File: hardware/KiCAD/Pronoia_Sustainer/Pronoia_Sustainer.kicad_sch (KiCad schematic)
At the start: 0 parts

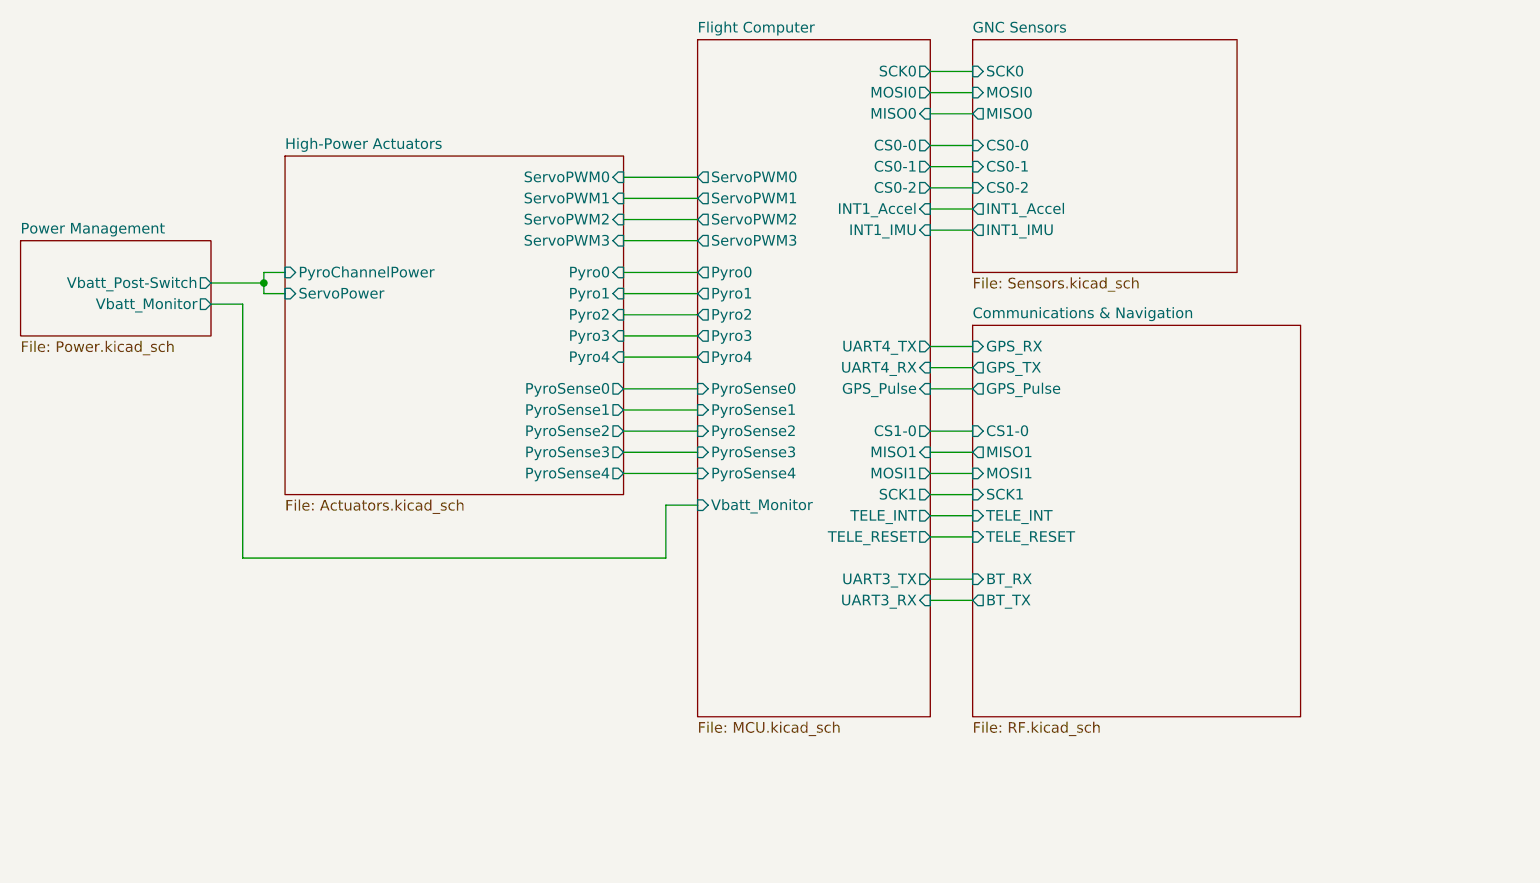
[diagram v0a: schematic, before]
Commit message: updated Schematics
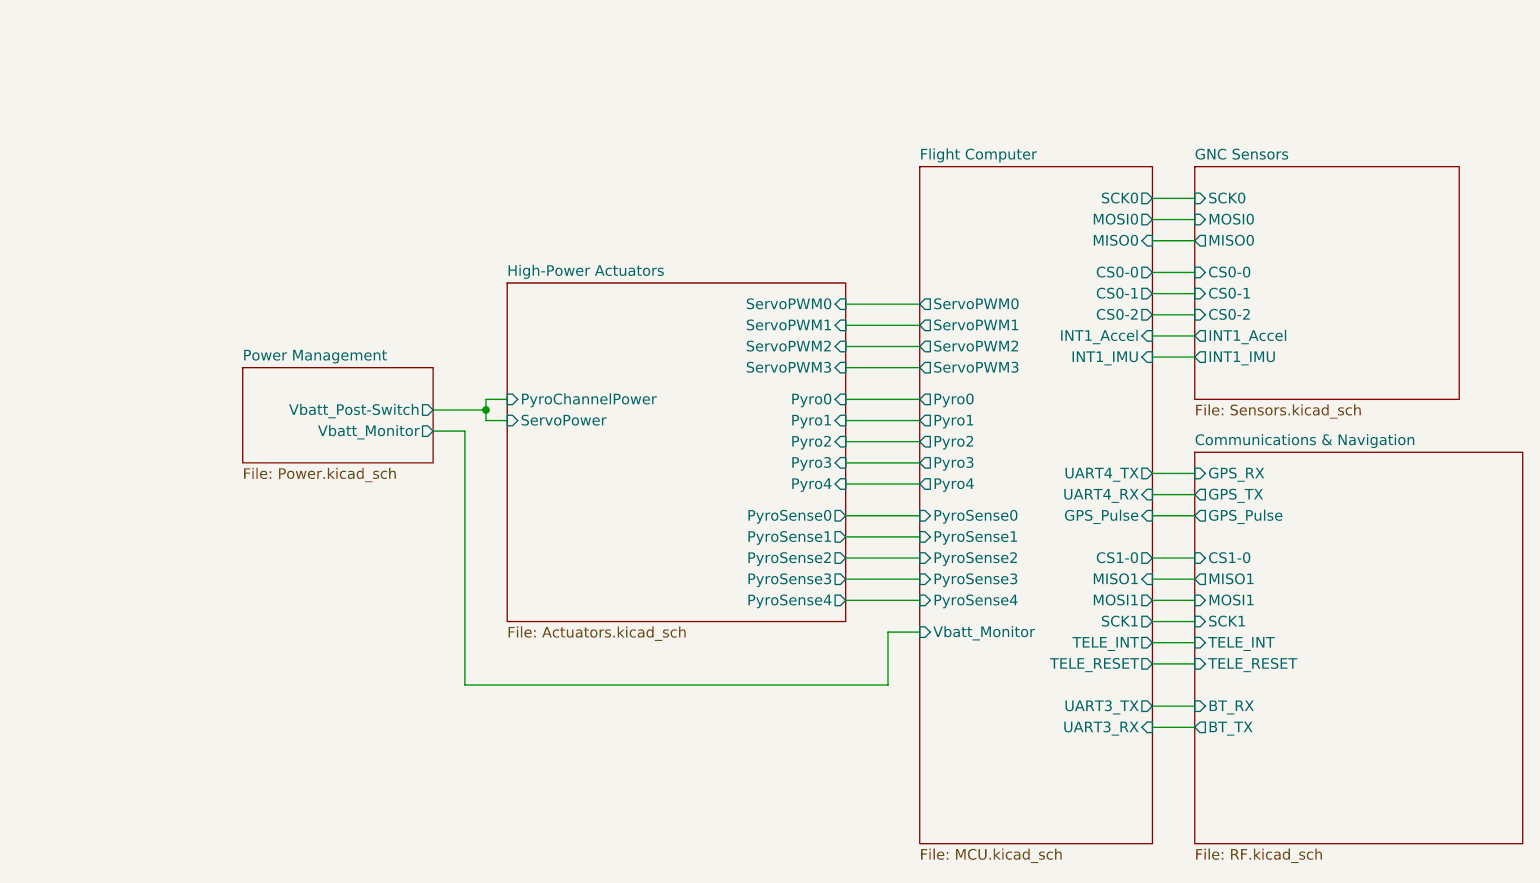
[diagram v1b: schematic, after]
